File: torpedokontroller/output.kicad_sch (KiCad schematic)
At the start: 36 parts, among them IC1 NCP81296MNTXG, IC9 TCAN3414DR, J1 64900411122, Q2 SiS443DN, Q6 PMOS, Q8 STANDARD_140356145200

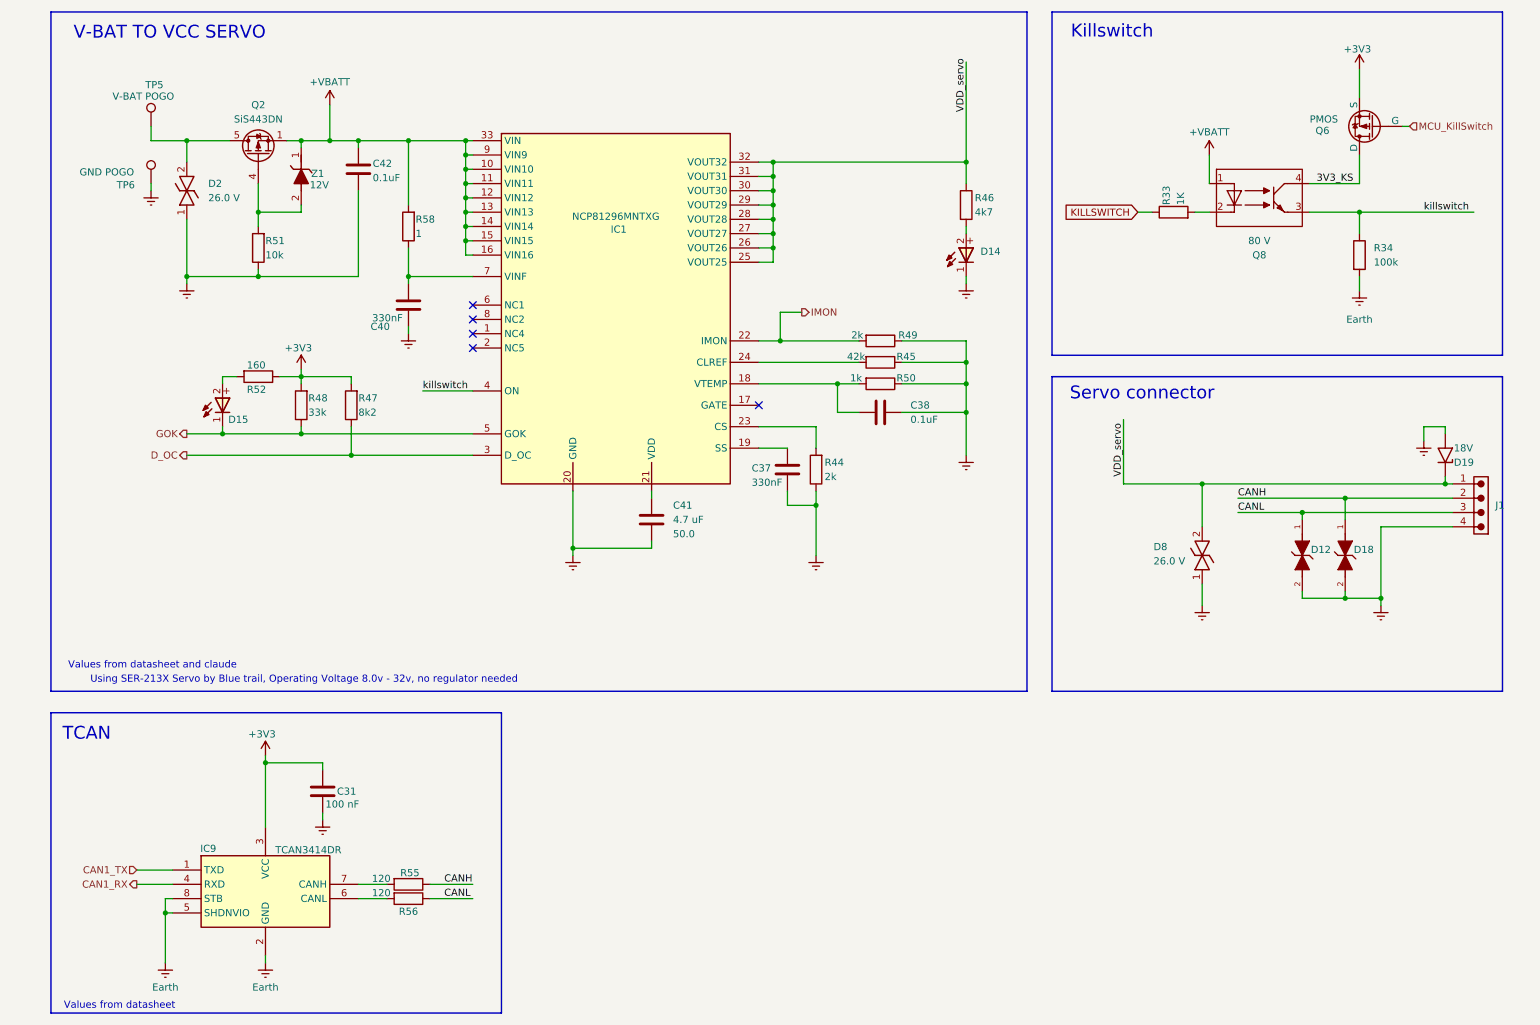
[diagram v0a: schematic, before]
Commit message: v 1.0
Ferdigish

CAN tvs-packages
Ground hook
Test pads
fixed some i/o issues
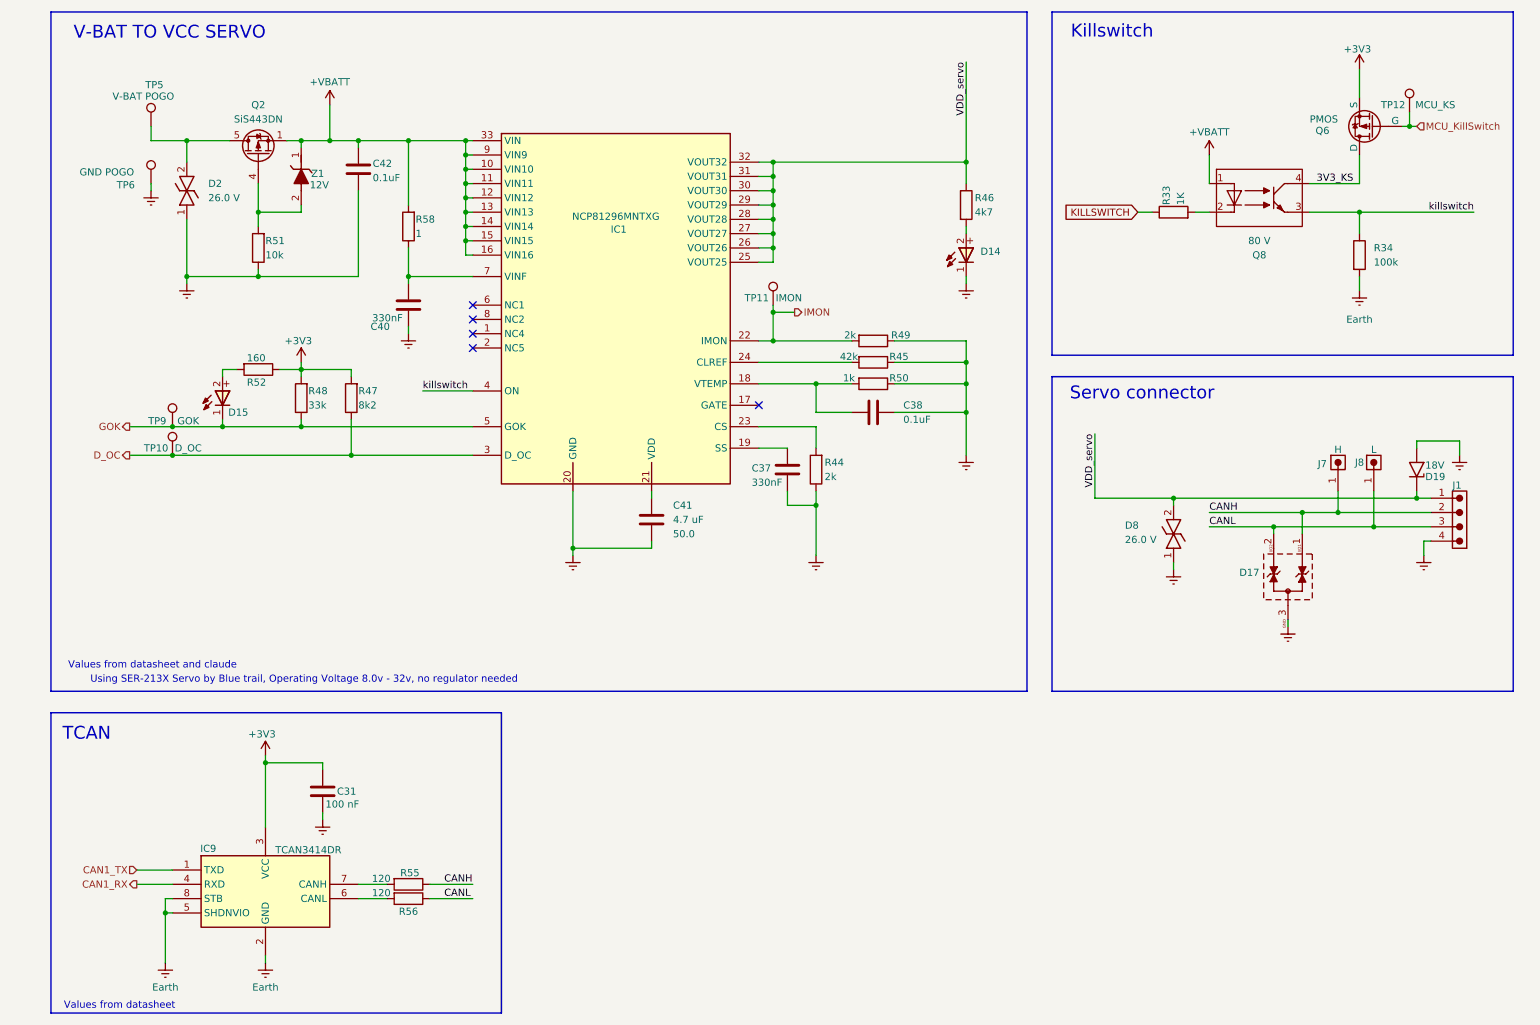
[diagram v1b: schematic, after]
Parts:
- removed D12, D18: WE-VE_0603, WE-VE_0603:WE-VE_0603, symbol WE-VE_0603:WE-VE_0603
- added D17: SOT23-3L_824094024, Diode_SMD_Wurth:D_Wurth_WE-TVS-SOT23-3L, symbol Diode_Wurth_WE-TVSP:SOT23-3L_824094024
- added J7: H, Connector_THT_Wurth:J_Wurth_WR-PHD_61300111121, symbol Connector_Wurth_WR-PHD:61300111121
- added J8: L, Connector_THT_Wurth:J_Wurth_WR-PHD_61300111121, symbol Connector_Wurth_WR-PHD:61300111121
- added TP10, TP11, TP12, TP9: TestPoint, TestPoint:TestPoint_Pad_D1.5mm, symbol Connector:TestPoint
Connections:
- net CANH: now also D17.1 (I/O1), J7.1
- net CANL: now also D17.2 (I/O2), J8.1
- net D_OC: now also TP10.1
- net Earth: now also D17.3 (GND)
- net GOK: now also TP9.1
- net IMON: now also TP11.1
- net MCU_KillSwitch: now also TP12.1
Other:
- moved on the sheet: C38, D15, D19, D8, J1, R45, R47, R48, R49, R50, R52
